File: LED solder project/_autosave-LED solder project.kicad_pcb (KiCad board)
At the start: 2 copper layers, 27.2 x 29.8 mm, 13 parts, among them Q1 PN2222A, SW1 SW_SPST

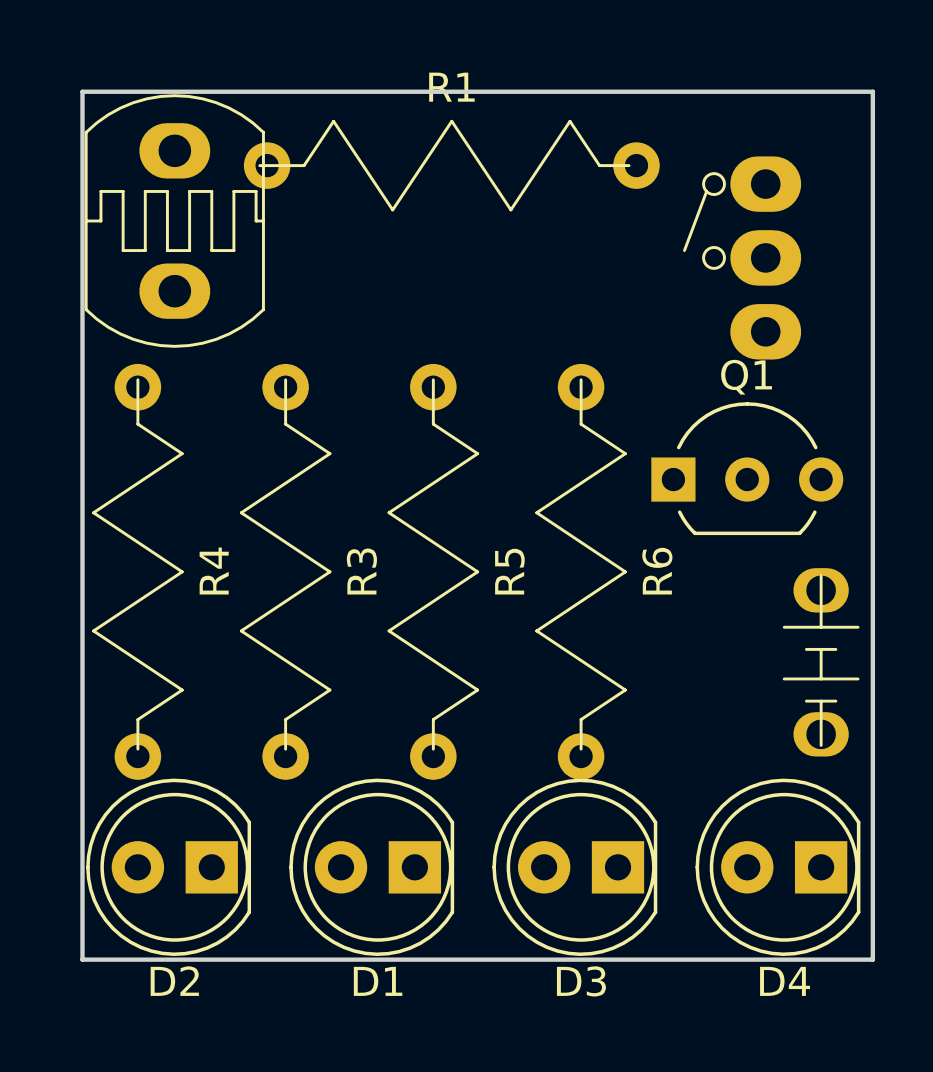
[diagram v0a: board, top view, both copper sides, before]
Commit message: added many
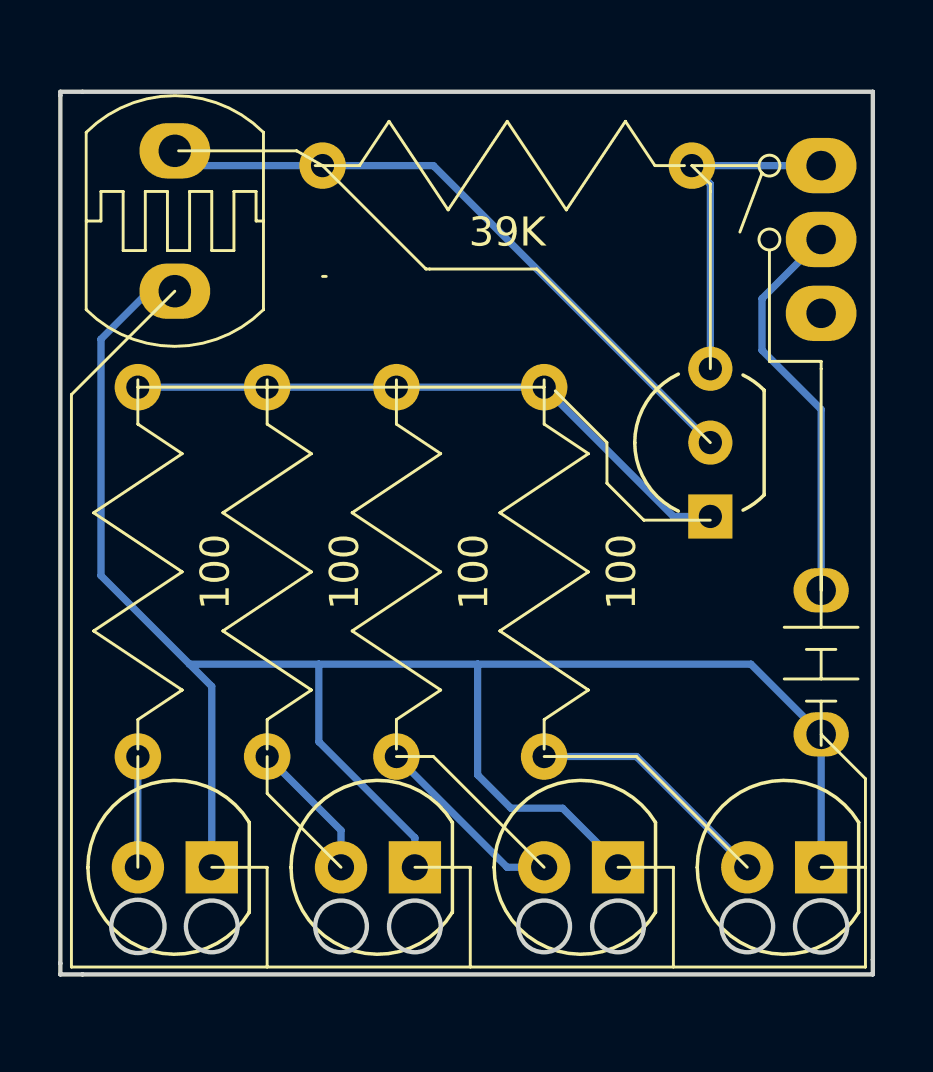
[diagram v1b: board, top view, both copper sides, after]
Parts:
- D1, D2, D3, D4: footprint LEDs:LED_D5.0mm -> rocketlib:LED
- Q1: footprint TO_SOT_Packages_THT:TO-92_Inline_Wide -> rocketlib:transistor
- moved SW1 2.01 mm to (152.4, 113.0)
- moved 39K 1.91 mm to (135.3, 110.5)
- moved Q1 1.80 mm to (148.6, 122.6), turned to 90 degrees
- moved 100 1.27 mm to (137.8, 118.1)
- moved 100 1.27 mm to (142.9, 118.1)
- moved 100 0.64 mm to (133.3, 118.1)
- renumbered R3 to 100, R4 to 100, R5 to 100, R6 to 100, R1 to 39K
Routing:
- net GND: track 0.00 -> 68.9 mm
- net Net-(Q1-Pad2): track 0.00 -> 22.6 mm
- net Net-(Q1-Pad1): track 0.00 -> 21.5 mm
- net VCC: track 0.00 -> 13.7 mm
- net Net-(Q1-Pad3): track 0.00 -> 11.7 mm
- net Net-(D4-Pad2): track 0.00 -> 8.56 mm
- net Net-(D3-Pad2): track 0.00 -> 6.66 mm
- net Net-(D1-Pad2): track 0.00 -> 4.86 mm
- net Net-(D2-Pad2): track 0.00 -> 3.81 mm
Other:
- board size 27.2 x 29.8 mm -> 27.9 x 30.4 mm
- board text added: "Designed by Collin Pearce"
